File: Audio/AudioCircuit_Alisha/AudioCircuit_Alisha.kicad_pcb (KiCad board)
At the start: 2 copper layers, 17 parts, among them J1 Conn_01x02_Pin, J2 PWM_VOL, J3 226Hz, U1 LM4875M, U4 TLV172IDCK

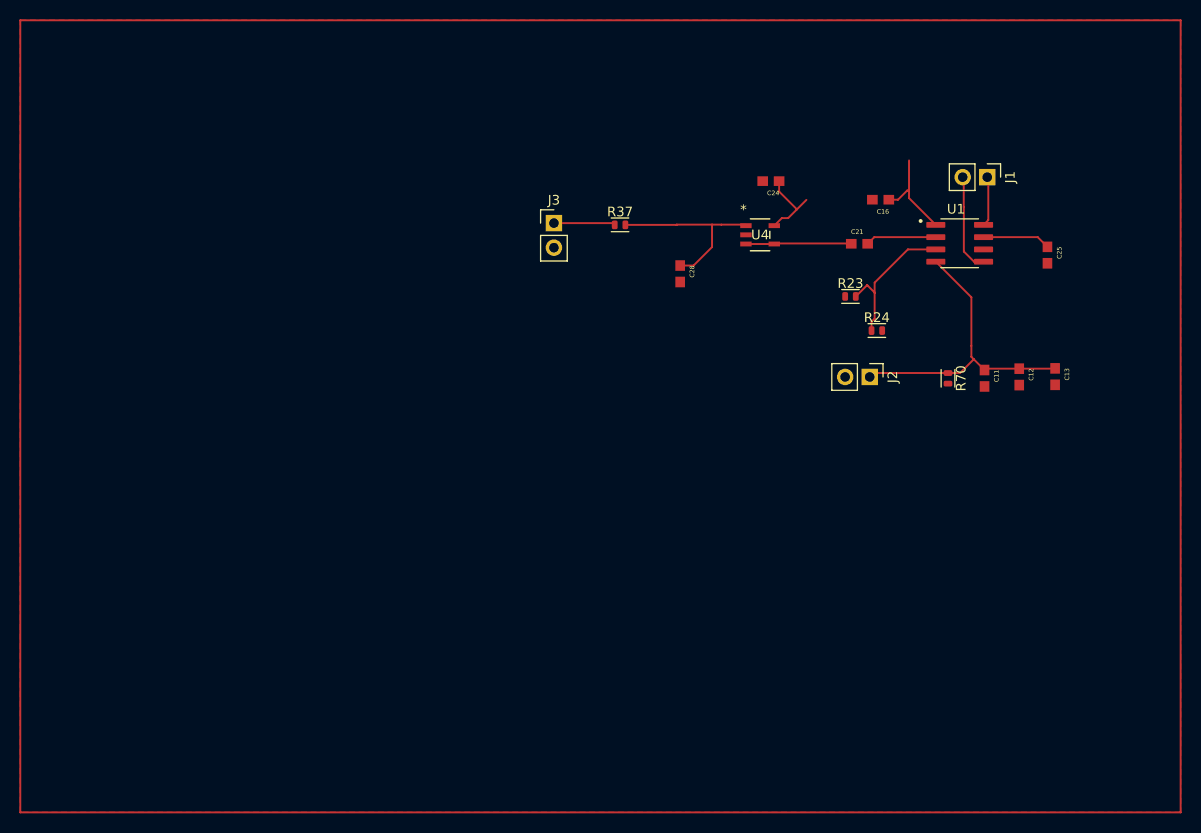
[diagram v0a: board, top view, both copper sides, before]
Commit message: audio circuit saved updates
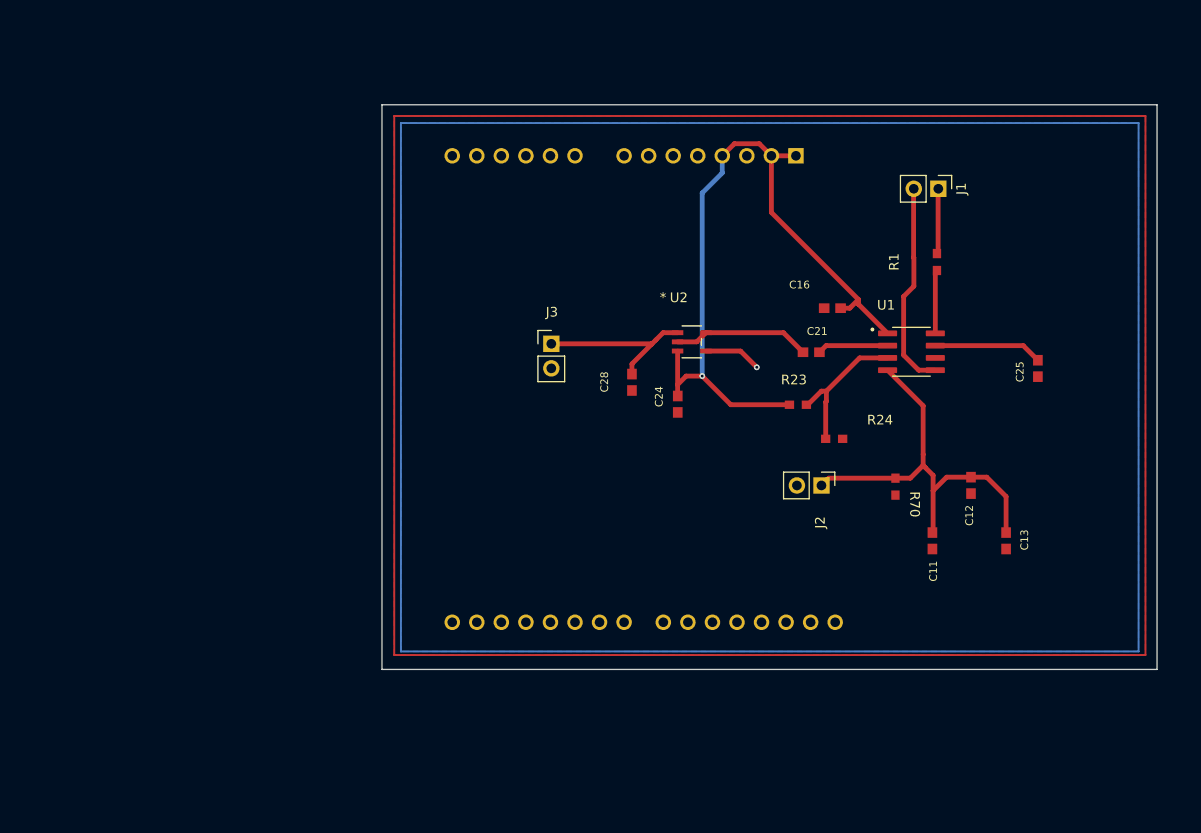
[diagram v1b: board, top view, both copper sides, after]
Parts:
- removed R37: 6.8k, Inductor_SMD:L_Changjiang_FTC160808S
- removed U4: TLV172IDCK, OP_AMP:DBV5_TEX-M
- added A1: Arduino_UNO_R2, Module:Arduino_UNO_R2, B.Cu at (191.5, 61.7)
- added R1: 300, Resistor1.60x0.80:RC0603N_YAG-M, F.Cu at (206.1, 72.7)
- added U2: ~, OP_AMP:DBV5_TEX-M, F.Cu at (180.7, 80.9)
- R23, R24, R70: footprint Inductor_SMD:L_Changjiang_FTC160808S -> Resistor1.60x0.80:RC0603N_YAG-M
- moved C24 25.0 mm to (179.3, 87.4), turned to -90 degrees
- moved C13 17.7 mm to (213.2, 101.5)
- moved C11 17.7 mm to (205.6, 101.5)
- moved J3 12.5 mm to (166.2, 81.1)
- moved R23 12.5 mm to (191.7, 87.4)
- moved R70 12.5 mm to (201.8, 95.9)
- moved C16 12.3 mm to (195.3, 77.4)
- moved C21 12.3 mm to (193.1, 82.0)
- moved C12 12.3 mm to (209.6, 95.8)
- moved C28 12.3 mm to (174.5, 85.1)
- moved J2 12.3 mm to (194.2, 95.8)
- moved U1 12.3 mm to (203.5, 82.0)
- moved R24 12.0 mm to (195.5, 91.0)
- moved C25 11.8 mm to (216.5, 83.7)
- moved J1 5.20 mm to (206.2, 65.1)
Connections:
- C28 pad 1: Net-(U4-+) -> Net-(J3-Pin_1)
- U1 pad 8: Net-(J1-Pin_1) -> Net-(U1-VO2)
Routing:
- net +3.3V: track 18.4 -> 75.7 mm, vias 0 -> 1
- net Net-(U4-+): track 18.9 -> 0.00 mm
- net Net-(J1-Pin_2): track 10.2 -> 21.6 mm
- net Net-(J3-Pin_1): track 6.36 -> 17.5 mm
- net Net-(J2-Pin_1): track 33.0 -> 43.1 mm
- net Net-(U1-VO2): track 0.00 -> 6.57 mm
- net GND: track 0.00 -> 5.96 mm, vias 0 -> 1
- net Net-(U1-BYPASS): track 7.18 -> 11.2 mm
- net Net-(U2--): track 10.9 -> 14.2 mm
- net Net-(J1-Pin_1): track 5.18 -> 6.76 mm
- added copper zone on B.Cu, net GND
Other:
- board outline added: 80.2 x 58.4 mm
